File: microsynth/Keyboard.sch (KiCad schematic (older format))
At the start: 54 parts, among them J5 Conn_01x02_Male, Q1 BC182, Q2 BC182L, SW1-DRIFT1 DRIFT, SW9 TRIGGER, U1 RC4136, U2 TL072, U3 4011, U4 4016, U5 LF347, U6 TL071

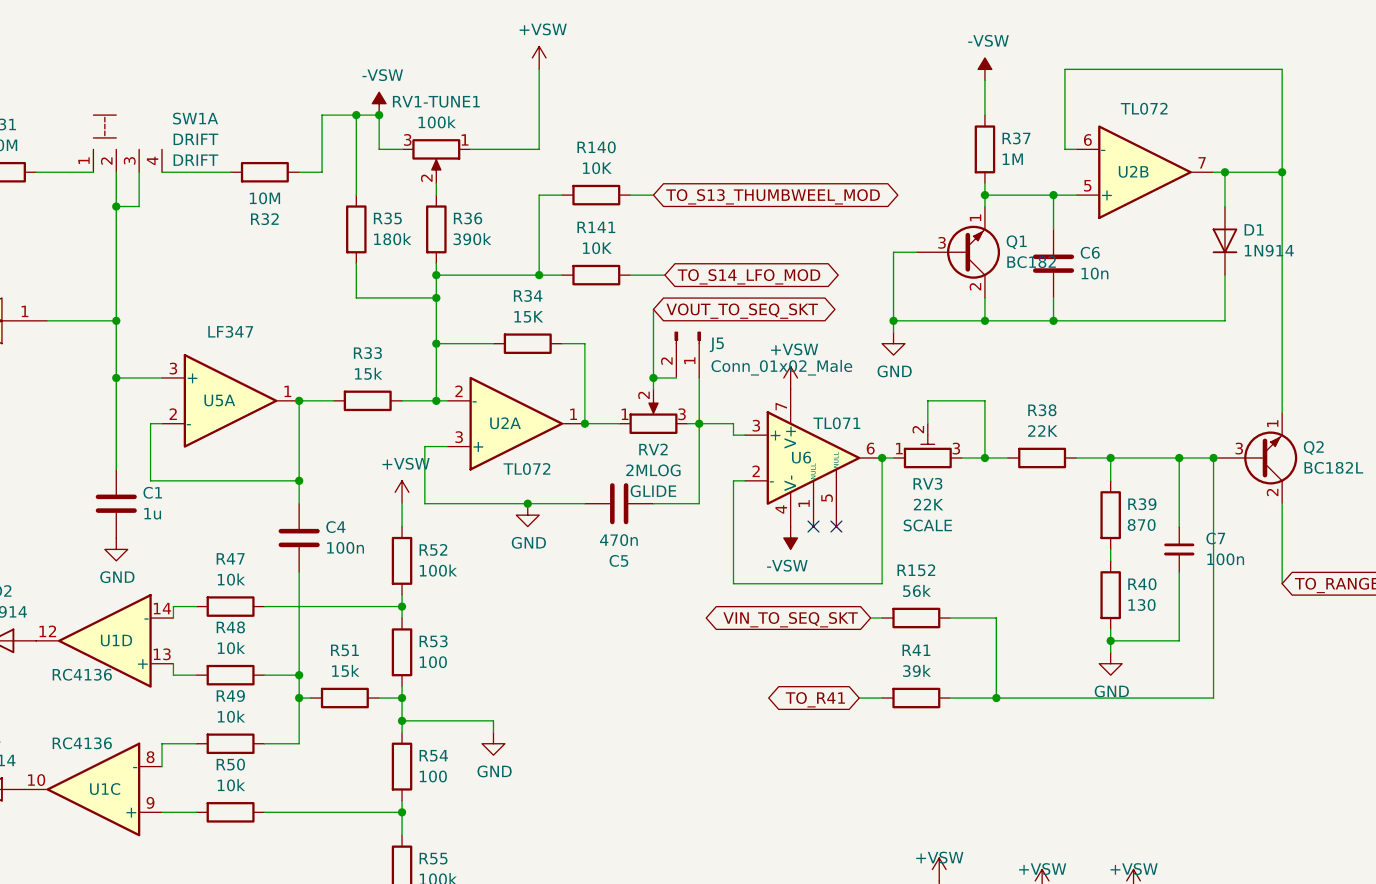
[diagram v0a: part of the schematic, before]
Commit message: Layout...
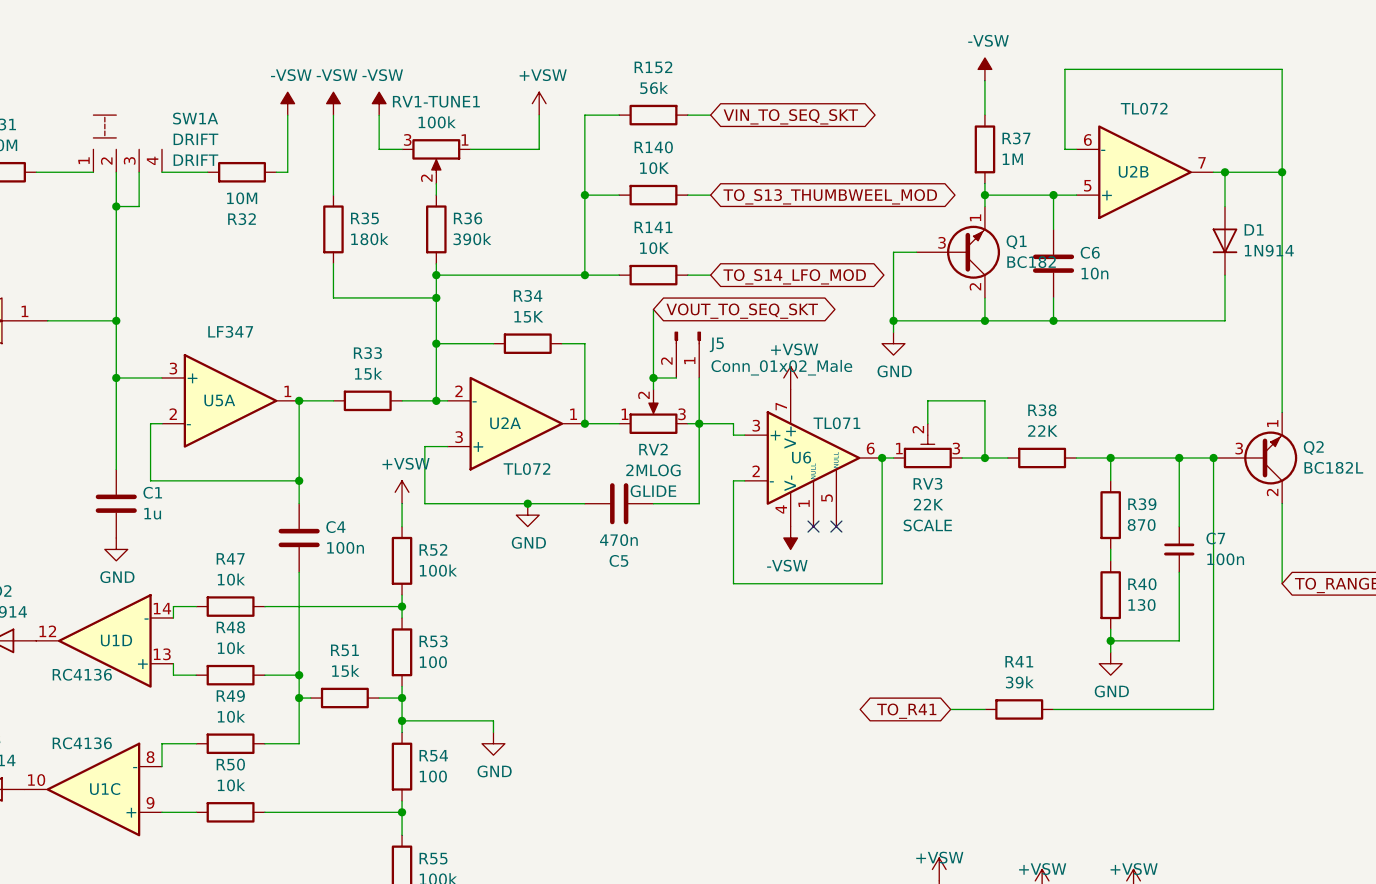
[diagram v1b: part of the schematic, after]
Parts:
- SW1-DRIFT1: footprint Buttons_Switches_ThroughHole:DP3T_Toggle -> Buttons_Switches_ThroughHole:OS203013MT8QN1
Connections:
- net at C7.1, Q2.3 (B), R38.1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: no longer R152.1
- net at R140.2, R141.2, R33.1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: now also R152.1
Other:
- moved on the sheet: R140, R141, R152, R32, R35, R41
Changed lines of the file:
@@
 F 0 "SW1" H 5844 1083 50  0000 L CNN
 F 1 "DRIFT" H 5844 992 50  0000 L CNN
-F 2 "Buttons_Switches_ThroughHole:DP3T_Toggle" H 5650 1050 50  0001 C CNN
-F 3 "" H 5650 1050 50  0001 C CNN
+F 2 "Buttons_Switches_ThroughHole:OS203013MT8QN1" H 5650 1050 50  0001 C CNN
+F 3 "https://www.tme.eu/Document/aa2d40399ed88e2cc02320a01dfb97ce/OSseries.pdf" H 5650 1050 50  0001 C CNN
 F 4 "DRIFT" H 5844 901 50  0000 L CNN "Label"
 	1    5650 1050
@@
 L Device:R R32
 U 1 1 5E9262E1
-P 6250 1250
-F 0 "R32" V 6043 1250 50  0000 C CNN
-F 1 "10M" V 6134 1250 50  0000 C CNN
-F 2 "Resistor_THT:R_Axial_DIN0207_L6.3mm_D2.5mm_P10.16mm_Horizontal" V 6180 1250 50  0001 C CNN
-F 3 "~" H 6250 1250 50  0001 C CNN
-	1    6250 1250
+P 6150 1250
+F 0 "R32" V 5943 1250 50  0000 C CNN
+F 1 "10M" V 6034 1250 50  0000 C CNN
+F 2 "Resistor_THT:R_Axial_DIN0207_L6.3mm_D2.5mm_P10.16mm_Horizontal" V 6080 1250 50  0001 C CNN
+F 3 "~" H 6150 1250 50  0001 C CNN
+	1    6150 1250
 	0    1    -1   0
 $EndComp
 Wire Wire Line
-	6100 1250 5800 1250
+	6000 1250 5800 1250
 $Comp
 L power:-VSW #PWR0208
@@
 $EndComp
 Wire Wire Line
-	6750 1000 6650 1000
-Wire Wire Line
-	6500 1000 6500 1250
-Wire Wire Line
-	6500 1250 6400 1250
+	6350 1000 6350 1250
+Wire Wire Line
+	6350 1250 6300 1250
 $Comp
 L Device:R R35
 U 1 1 5E930BCA
-P 6650 1500
-F 0 "R35" H 6720 1546 50  0000 L CNN
-F 1 "180k" H 6720 1455 50  0000 L CNN
-F 2 "Resistor_THT:R_Axial_DIN0207_L6.3mm_D2.5mm_P10.16mm_Horizontal" V 6580 1500 50  0001 C CNN
-F 3 "~" H 6650 1500 50  0001 C CNN
-	1    6650 1500
+P 6550 1500
+F 0 "R35" H 6620 1546 50  0000 L CNN
+F 1 "180k" H 6620 1455 50  0000 L CNN
+F 2 "Resistor_THT:R_Axial_DIN0207_L6.3mm_D2.5mm_P10.16mm_Horizontal" V 6480 1500 50  0001 C CNN
+F 3 "~" H 6550 1500 50  0001 C CNN
+	1    6550 1500
 	1    0    0    -1
 $EndComp
@@
 	7000 2250 7000 2000
 Wire Wire Line
-	6650 1650 6650 1800
-Wire Wire Line
-	6650 1800 7000 1800
+	6550 1650 6550 1800
+Wire Wire Line
+	6550 1800 7000 1800
 Connection ~ 7000 1800
 Wire Wire Line
@@
 Wire Wire Line
 	6750 1150 6750 1000
-Connection ~ 6750 1000
-Wire Wire Line
-	6650 1350 6650 1000
-Connection ~ 6650 1000
-Wire Wire Line
-	6650 1000 6500 1000
+Wire Wire Line
+	6550 1350 6550 1000
 Wire Wire Line
 	7000 1300 7000 1350
@@
 L power:+VSW #PWR0209
 U 1 1 5E93EA0A
-P 7450 800
-F 0 "#PWR0209" H 7450 650 50  0001 C CNN
-F 1 "+VSW" H 7465 973 50  0000 C CNN
-F 2 "" H 7450 800 50  0001 C CNN
-F 3 "" H 7450 800 50  0001 C CNN
-	1    7450 800
-	1    0    0    -1
-$EndComp
-Wire Wire Line
-	7450 800  7450 1150
+P 7450 1000
+F 0 "#PWR0209" H 7450 850 50  0001 C CNN
+F 1 "+VSW" H 7465 1173 50  0000 C CNN
+F 2 "" H 7450 1000 50  0001 C CNN
+F 3 "" H 7450 1000 50  0001 C CNN
+	1    7450 1000
+	1    0    0    -1
+$EndComp
+Wire Wire Line
+	7450 1000 7450 1150
 Wire Wire Line
 	7450 1150 7150 1150
@@
 L Device:R R140
 U 1 1 5E940A1E
-P 7700 1350
-F 0 "R140" V 7493 1350 50  0000 C CNN
-F 1 "10K" V 7584 1350 50  0000 C CNN
-F 2 "Resistor_THT:R_Axial_DIN0207_L6.3mm_D2.5mm_P10.16mm_Horizontal" V 7630 1350 50  0001 C CNN
-F 3 "~" H 7700 1350 50  0001 C CNN
-	1    7700 1350
+P 7950 1350
+F 0 "R140" V 7743 1350 50  0000 C CNN
+F 1 "10K" V 7834 1350 50  0000 C CNN
+F 2 "Resistor_THT:R_Axial_DIN0207_L6.3mm_D2.5mm_P10.16mm_Horizontal" V 7880 1350 50  0001 C CNN
+F 3 "~" H 7950 1350 50  0001 C CNN
+	1    7950 1350
 	0    1    1    0
 $EndComp
@@
 L Device:R R141
 U 1 1 5E941296
-P 7700 1700
-F 0 "R141" V 7493 1700 50  0000 C CNN
-F 1 "10K" V 7584 1700 50  0000 C CNN
-F 2 "Resistor_THT:R_Axial_DIN0207_L6.3mm_D2.5mm_P10.16mm_Horizontal" V 7630 1700 50  0001 C CNN
-F 3 "~" H 7700 1700 50  0001 C CNN
-	1    7700 1700
-	0    1    1    0
-$EndComp
-Wire Wire Line
-	7550 1700 7450 1700
+P 7950 1700
+F 0 "R141" V 7743 1700 50  0000 C CNN
+F 1 "10K" V 7834 1700 50  0000 C CNN
+F 2 "Resistor_THT:R_Axial_DIN0207_L6.3mm_D2.5mm_P10.16mm_Horizontal" V 7880 1700 50  0001 C CNN
+F 3 "~" H 7950 1700 50  0001 C CNN
+	1    7950 1700
+	0    1    1    0
+$EndComp
+Wire Wire Line
+	7800 1700 7650 1700
 Connection ~ 7000 1700
 Wire Wire Line
 	7000 1700 7000 1650
 Wire Wire Line
-	7450 1700 7450 1350
-Wire Wire Line
-	7450 1350 7550 1350
-Connection ~ 7450 1700
-Wire Wire Line
-	7450 1700 7000 1700
-Wire Wire Line
-	8000 1700 7850 1700
-Wire Wire Line
-	7950 1350 7850 1350
+	7650 1700 7650 1350
+Wire Wire Line
+	7650 1350 7800 1350
+Connection ~ 7650 1700
+Wire Wire Line
+	7650 1700 7000 1700
+Wire Wire Line
+	8200 1700 8100 1700
+Wire Wire Line
+	8200 1350 8100 1350
 $Comp
 L Device:R R34
@@
 L Device:R R152
 U 1 1 5E98598E
-P 9100 3200
-F 0 "R152" V 8893 3200 50  0000 C CNN
-F 1 "56k" V 8984 3200 50  0000 C CNN
-F 2 "Resistor_THT:R_Axial_DIN0207_L6.3mm_D2.5mm_P10.16mm_Horizontal" V 9030 3200 50  0001 C CNN
-F 3 "~" H 9100 3200 50  0001 C CNN
-	1    9100 3200
-	0    1    1    0
+P 7950 1000
+F 0 "R152" V 7743 1000 50  0000 C CNN
+F 1 "56k" V 7834 1000 50  0000 C CNN
+F 2 "Resistor_THT:R_Axial_DIN0207_L6.3mm_D2.5mm_P10.16mm_Horizontal" V 7880 1000 50  0001 C CNN
+F 3 "~" H 7950 1000 50  0001 C CNN
+	1    7950 1000
+	0    -1   1    0
 $EndComp
 $Comp
 L Device:R R41
 U 1 1 5E9860CB
-P 9100 3550
-F 0 "R41" V 8893 3550 50  0000 C CNN
-F 1 "39k" V 8984 3550 50  0000 C CNN
-F 2 "Resistor_THT:R_Axial_DIN0207_L6.3mm_D2.5mm_P10.16mm_Horizontal" V 9030 3550 50  0001 C CNN
-F 3 "~" H 9100 3550 50  0001 C CNN
-	1    9100 3550
-	0    1    1    0
-$EndComp
-Wire Wire Line
-	9250 3550 9450 3550
-Wire Wire Line
-	9450 3550 9450 3200
-Wire Wire Line
-	9450 3200 9250 3200
-Wire Wire Line
-	9450 3550 10400 3550
-Wire Wire Line
-	10400 3550 10400 2500
-Connection ~ 9450 3550
+P 9550 3600
+F 0 "R41" V 9343 3600 50  0000 C CNN
+F 1 "39k" V 9434 3600 50  0000 C CNN
+F 2 "Resistor_THT:R_Axial_DIN0207_L6.3mm_D2.5mm_P10.16mm_Horizontal" V 9480 3600 50  0001 C CNN
+F 3 "~" H 9550 3600 50  0001 C CNN
+	1    9550 3600
+	0    1    1    0
+$EndComp
+Wire Wire Line
+	7650 1350 7650 1000
+Wire Wire Line
+	7650 1000 7800 1000
+Wire Wire Line
+	10400 3600 10400 2500
 Connection ~ 10400 2500
 Wire Wire Line
-	8900 3200 8950 3200
-Wire Wire Line
-	8950 3550 8850 3550
+	8200 1000 8100 1000
+Wire Wire Line
+	9400 3600 9250 3600
 Wire Wire Line
 	6400 2700 6400 2600
@@
 Wire Wire Line
 	10700 2700 10700 3050
-Text GLabel 8850 3550 0    50   BiDi ~ 0
+Text GLabel 9250 3600 0    50   BiDi ~ 0
 TO_R41
-Text GLabel 7950 1350 2    50   BiDi ~ 0
+Text GLabel 8200 1350 2    50   BiDi ~ 0
 TO_S13_THUMBWEEL_MOD
-Text GLabel 8000 1700 2    50   BiDi ~ 0
+Text GLabel 8200 1700 2    50   BiDi ~ 0
 TO_S14_LFO_MOD
 Text GLabel 7950 1850 2    50   BiDi ~ 0
@@
 Text GLabel 3700 2800 2    50   BiDi ~ 0
 TRIG_OUT_TO_SEQ_SKT
-Text GLabel 8900 3200 0    50   BiDi ~ 0
+Text GLabel 8200 1000 2    50   BiDi ~ 0
 VIN_TO_SEQ_SKT
 Wire Wire Line
@@
 Wire Wire Line
 	8150 2150 8150 2350
+$Comp
+L power:-VSW #PWR0228
+U 1 1 5E98AA20
+P 6350 1000
+F 0 "#PWR0228" H 6350 1100 50  0001 C CNN
+F 1 "-VSW" H 6365 1173 50  0000 C CNN
+F 2 "" H 6350 1000 50  0001 C CNN
+F 3 "" H 6350 1000 50  0001 C CNN
+	1    6350 1000
+	1    0    0    -1
+$EndComp
+$Comp
+L power:-VSW #PWR0229
+U 1 1 5E98AE00
+P 6550 1000
+F 0 "#PWR0229" H 6550 1100 50  0001 C CNN
+F 1 "-VSW" H 6565 1173 50  0000 C CNN
+F 2 "" H 6550 1000 50  0001 C CNN
+F 3 "" H 6550 1000 50  0001 C CNN
+	1    6550 1000
+	1    0    0    -1
+$EndComp
+Connection ~ 7650 1350
+Wire Wire Line
+	9700 3600 10400 3600
 $EndSCHEMATC

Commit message: Layout...
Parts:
- SW1-DRIFT1: footprint Buttons_Switches_ThroughHole:OS203013MT8QN1 -> Buttons_Switches_ThroughHole:L203011MS02Q
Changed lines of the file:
@@
 F 0 "SW1" H 5844 1083 50  0000 L CNN
 F 1 "DRIFT" H 5844 992 50  0000 L CNN
-F 2 "Buttons_Switches_ThroughHole:OS203013MT8QN1" H 5650 1050 50  0001 C CNN
+F 2 "Buttons_Switches_ThroughHole:L203011MS02Q" H 5650 1050 50  0001 C CNN
 F 3 "https://www.tme.eu/Document/aa2d40399ed88e2cc02320a01dfb97ce/OSseries.pdf" H 5650 1050 50  0001 C CNN
 F 4 "DRIFT" H 5844 901 50  0000 L CNN "Label"
